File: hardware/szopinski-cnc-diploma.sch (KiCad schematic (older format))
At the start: 26 parts, among them J1 Barrel_Jack, J2 Conn_02x08_Odd_Even, J3 AVR-ISP-10, J4 Conn_01x04, J5 Conn_01x04, J6 Conn_01x04, J7 Conn_01x04, U1 ATmega328P-PU, U2 L7805, U3 DRV8825, U4 DRV8825, U5 DRV8825, U6 DRV8825, Y1 20 MHz

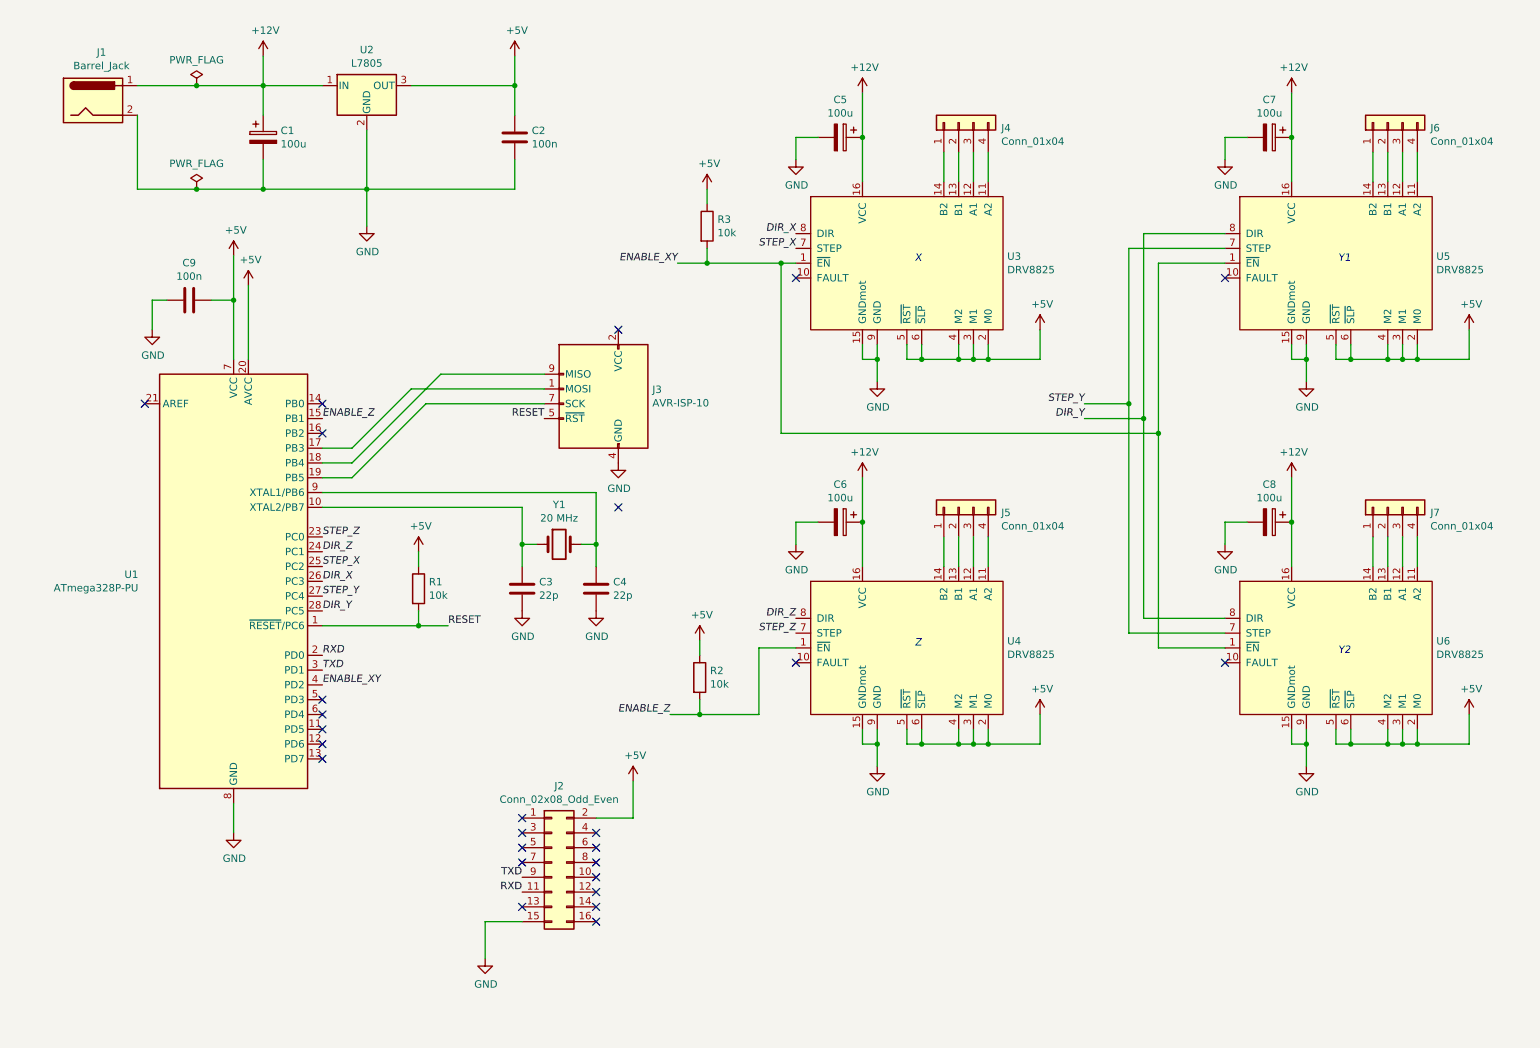
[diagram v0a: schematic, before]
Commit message: Advisor review
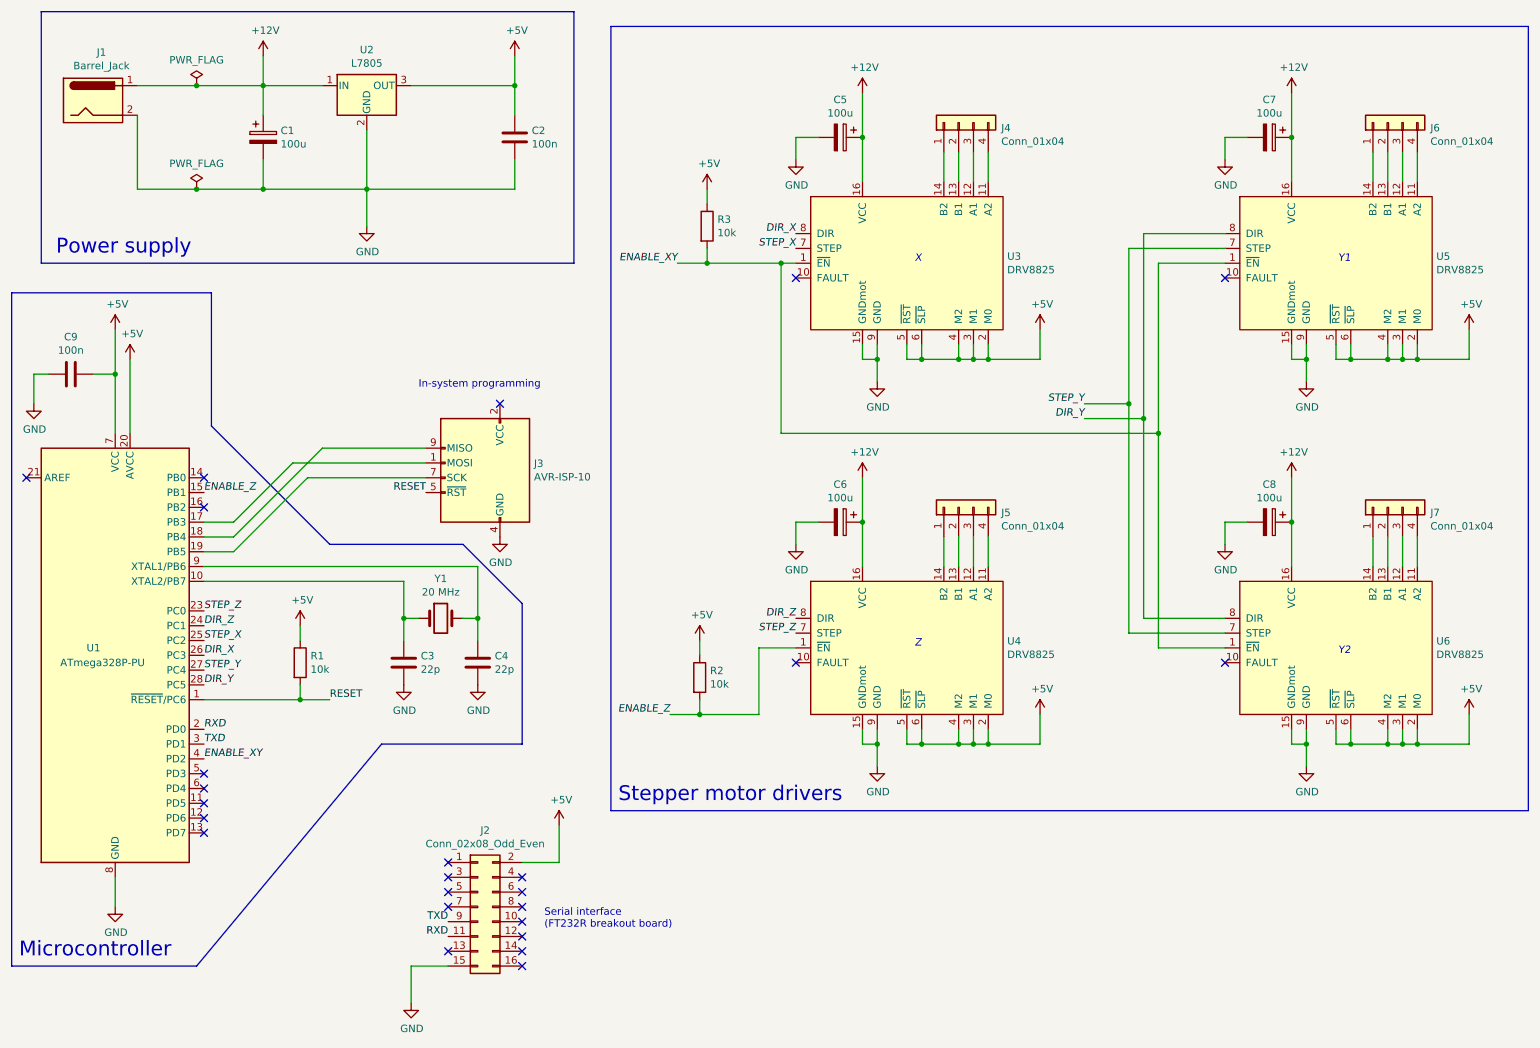
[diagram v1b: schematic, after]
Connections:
- no-connect marks 26 -> 25
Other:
- note added: "In-system programming"
- note added: "Microcontroller"
- note added: "Power supply"
- note added: "Serial interface\n(FT232R breakout board)"
- note added: "Stepper motor drivers"
- moved on the sheet: C3, C4, C9, J2, J3, R1, U1, Y1
